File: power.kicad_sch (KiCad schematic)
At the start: 18 parts, among them J3 Conn_01x02, Q1 Q_NMOS_SSSGD_AvalancheRated, U4 TPS25983, U5 LM74700, U7 AMS1117-3.3, U8 AMS1117-5.0

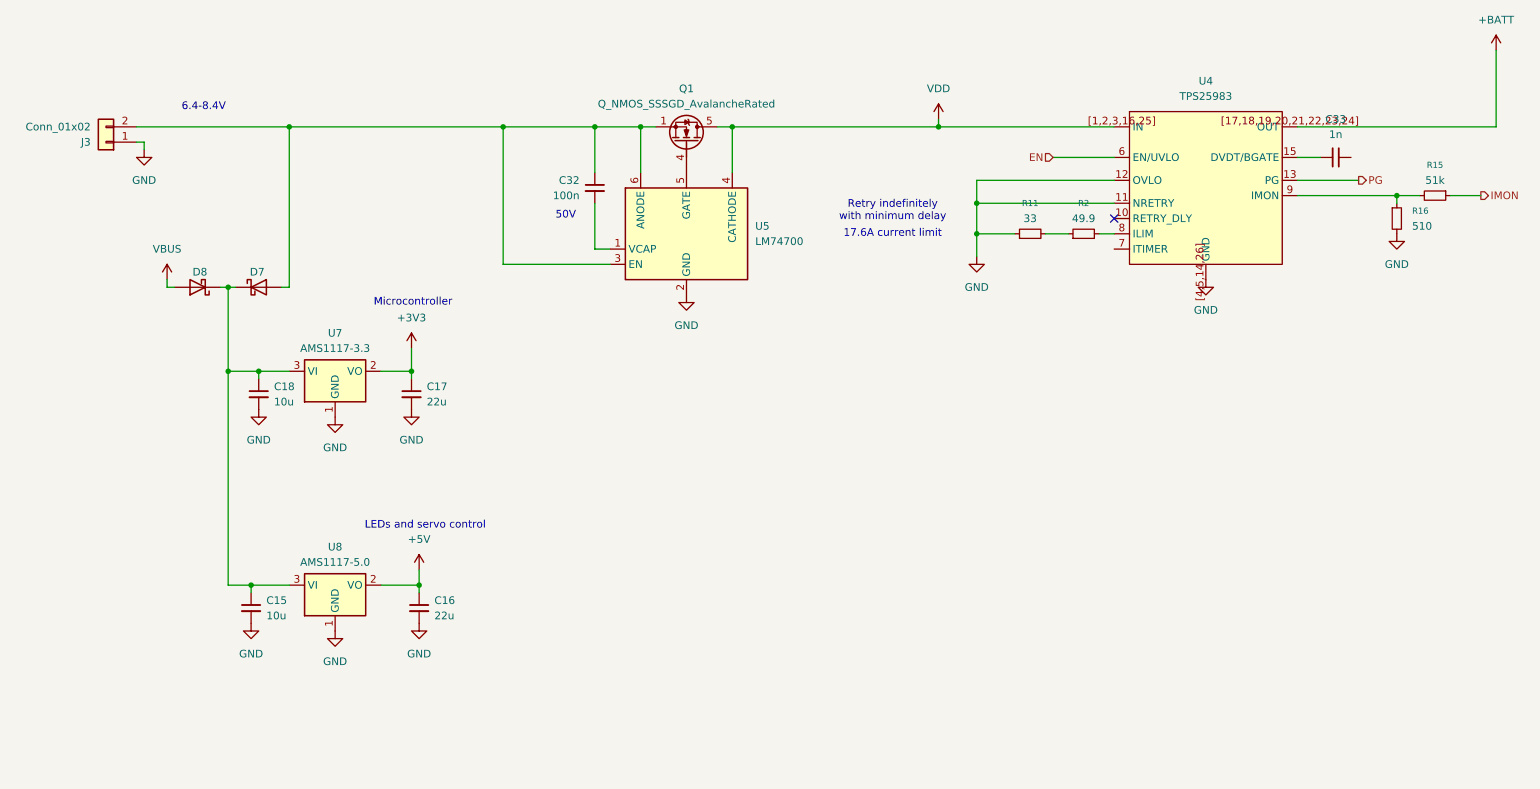
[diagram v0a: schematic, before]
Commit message: restore symbols library, wire up PG and IMON, refine routing
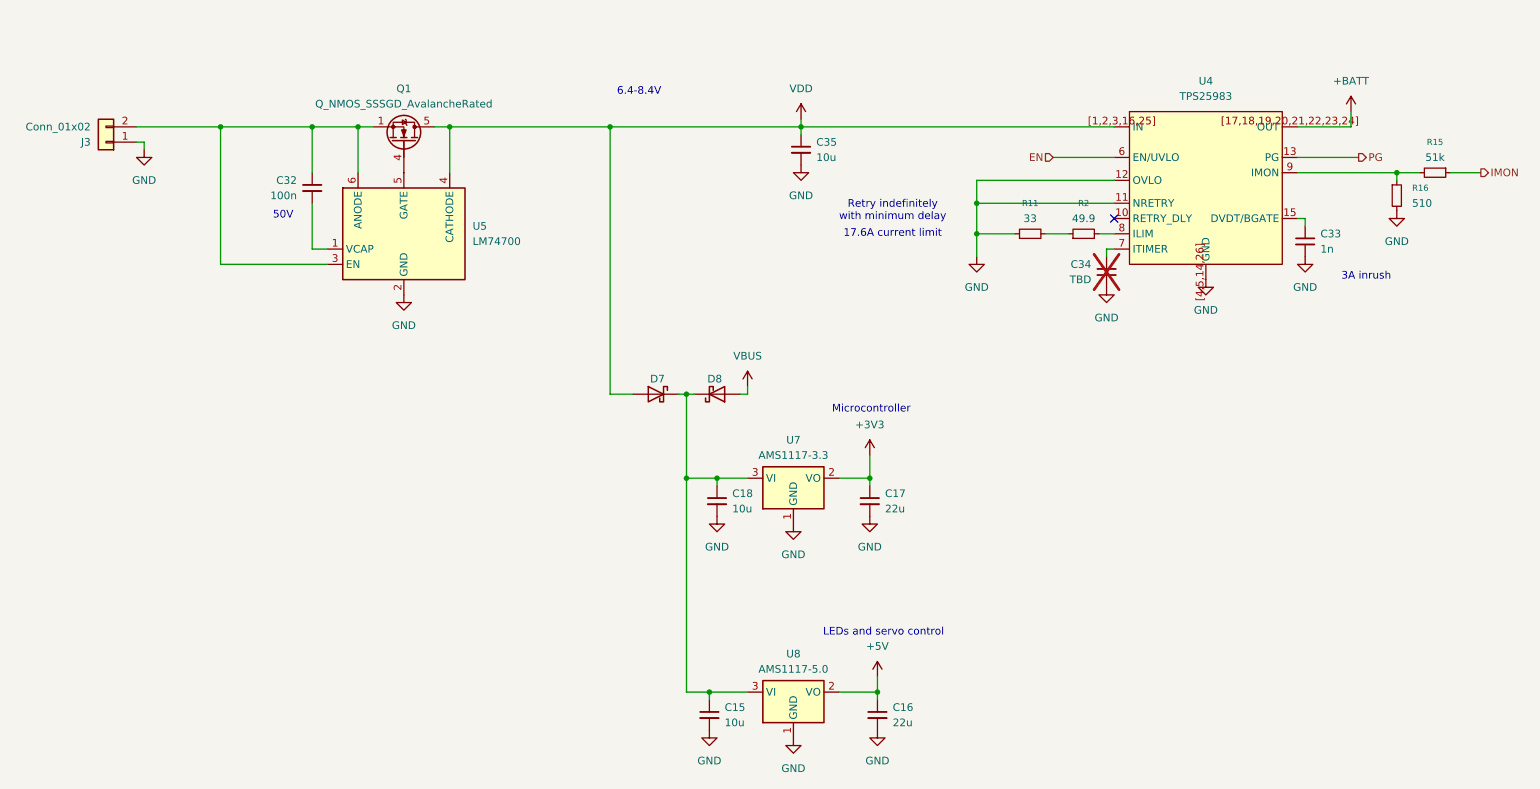
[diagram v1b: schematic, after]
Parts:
- added C34: TBD, Capacitor_SMD:C_0402_1005Metric, symbol Device:C_Small
- added C35: 10u, Capacitor_SMD:C_0603_1608Metric, symbol Device:C_Small
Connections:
- net GND: now also C33.1, C34.1, C35.2
- net VDD: now also D7.2 (A), C35.1
- net at C32.1, J3.2 (Pin_2), Q1.1 (S)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: no longer D7.2 (A)
- net at U4.15 (DVDT/BGATE): now also C33.2; no longer C33.1
- net at U4.7 (ITIMER): now also C34.2
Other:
- note added: "3A inrush"
- moved on the sheet: C15, C16, C17, C18, C32, D7, D8, Q1, R15, R16, U5, U7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
